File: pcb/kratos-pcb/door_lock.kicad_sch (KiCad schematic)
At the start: 8 parts, among them IC1 SN74HC595N, Q2 2N2222A, Q3 2N2222A, U2 74HC595

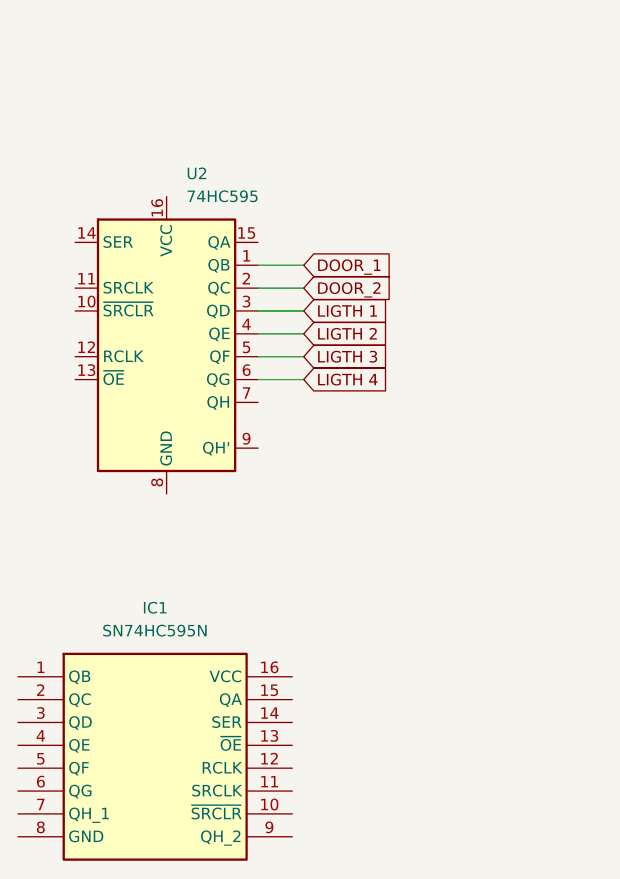
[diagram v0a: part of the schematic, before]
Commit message: ### added
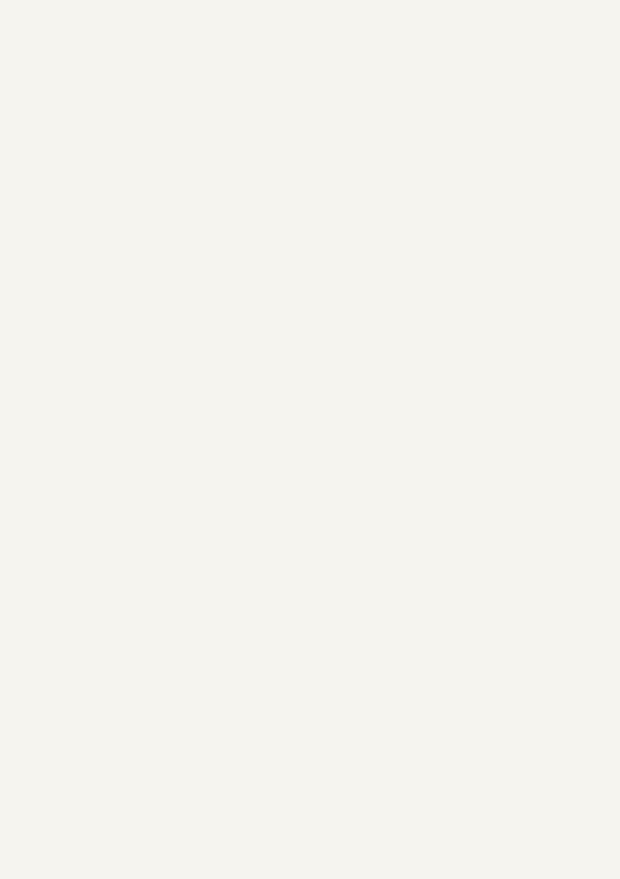
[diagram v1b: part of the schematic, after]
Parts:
- removed IC1: SN74HC595N, DIP794W53P254L1930H508Q16N, symbol SN74HC595N:SN74HC595N
- removed U2: 74HC595, symbol 74xx:74HC595

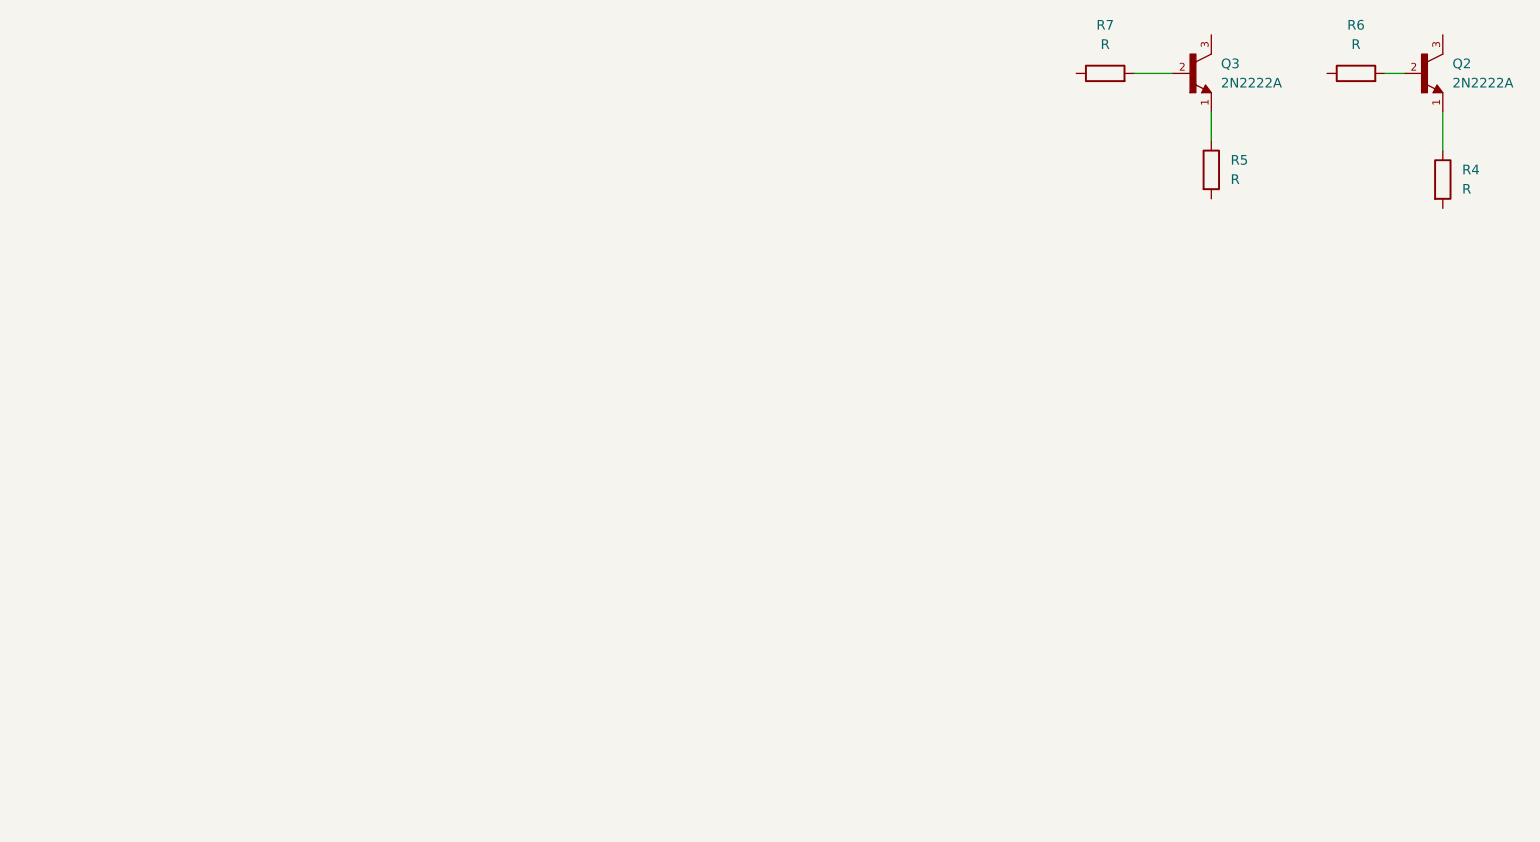
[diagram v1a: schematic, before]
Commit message: ### added
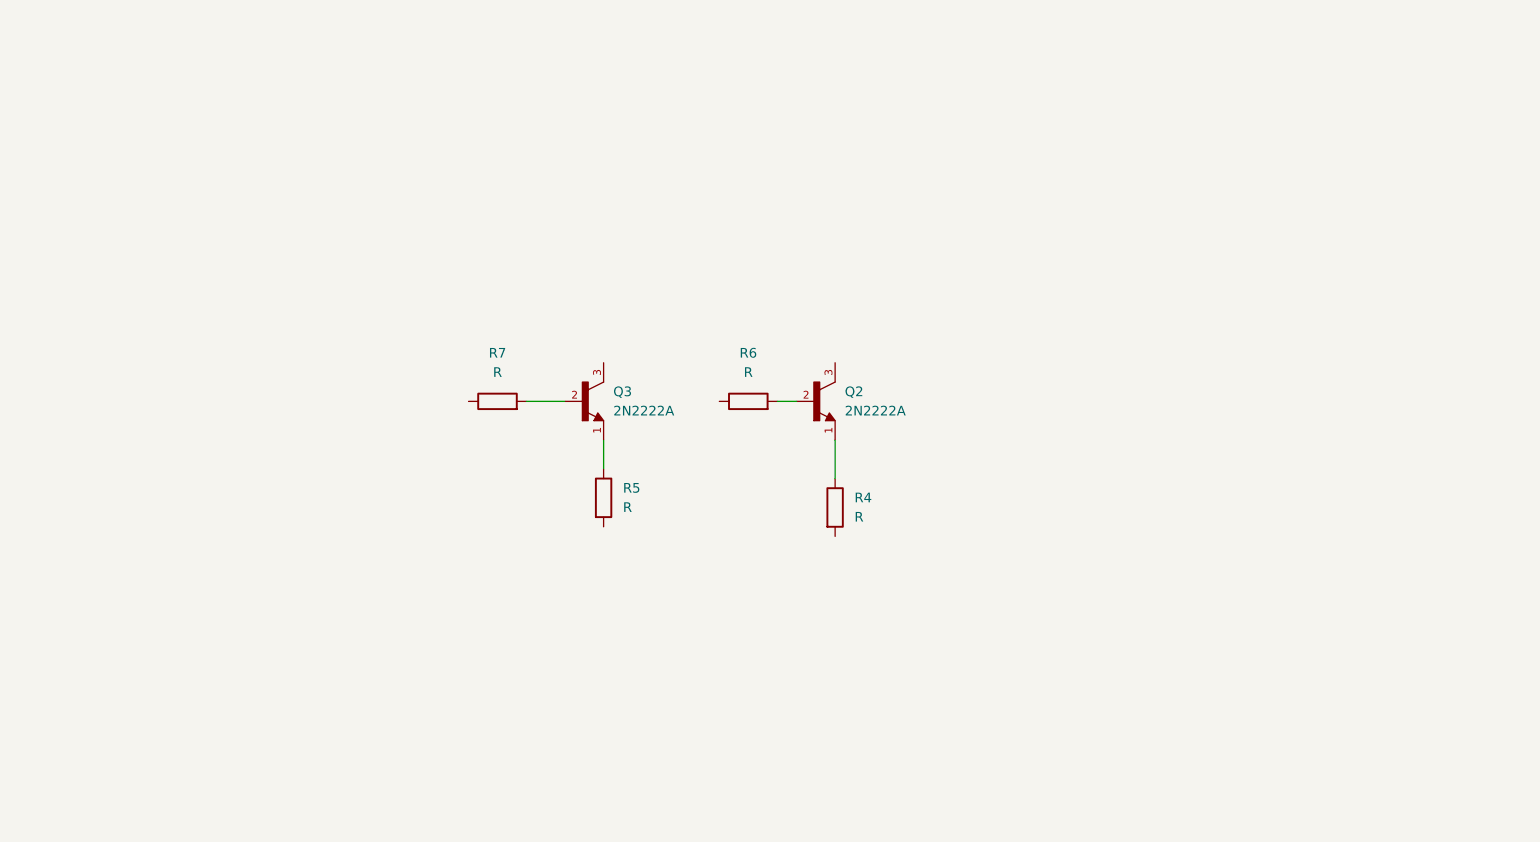
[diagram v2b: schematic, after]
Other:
- moved on the sheet: Q2, Q3, R4, R5, R6, R7

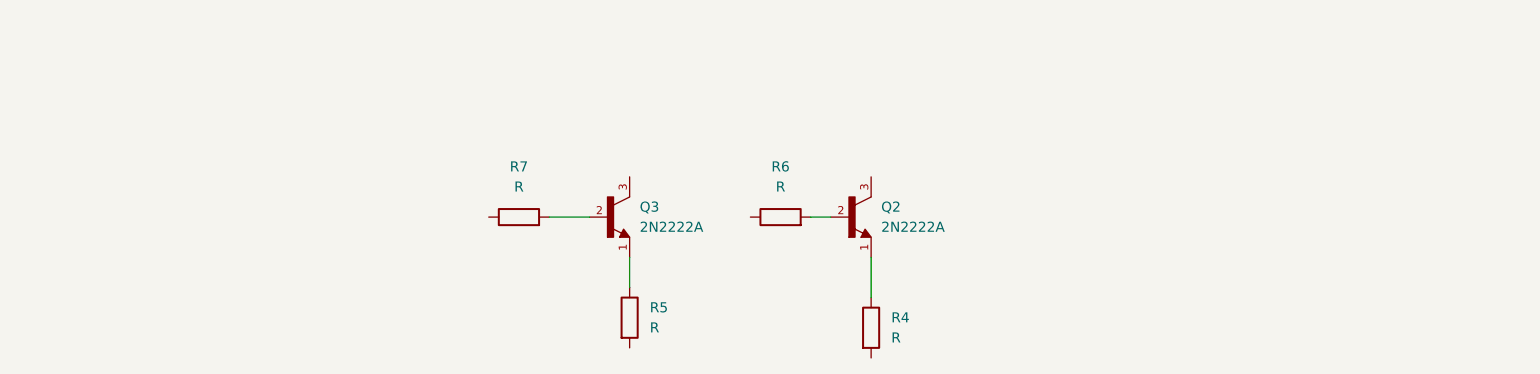
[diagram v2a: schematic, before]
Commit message: ### update     - kicad schematic
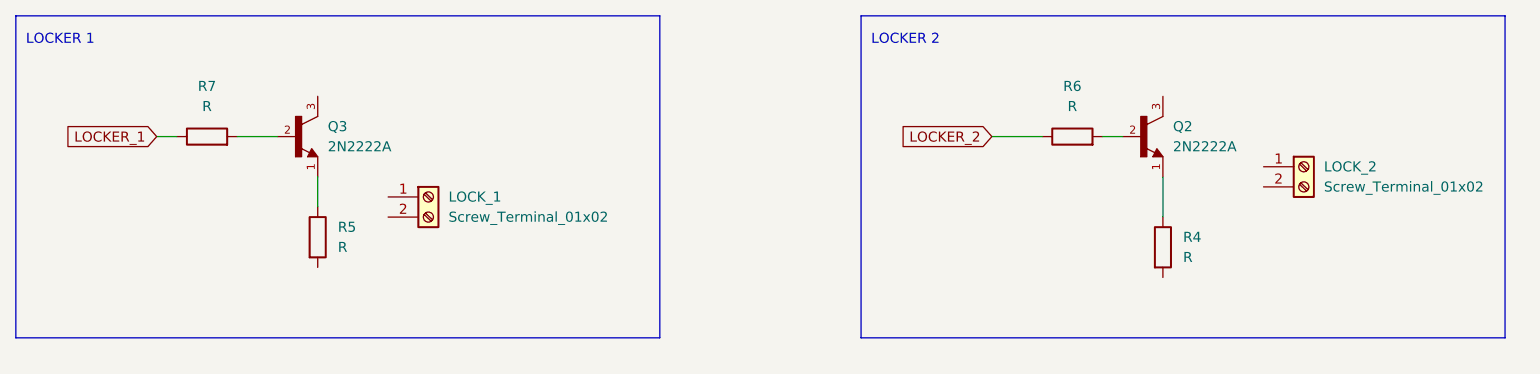
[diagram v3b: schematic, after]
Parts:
- added LOCK_1, LOCK_2: Screw_Terminal_01x02, TerminalBlock:TerminalBlock_bornier-2_P5.08mm, symbol Connector:Screw_Terminal_01x02
- R4, R5, R6, R7: footprint (none) -> Resistor_THT:R_Axial_DIN0204_L3.6mm_D1.6mm_P5.08mm_Horizontal
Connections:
- net LOCKER_2: now reaches R6.1
- net LOCKER_1: now reaches R7.1
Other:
- note added: "LOCKER 1"
- note added: "LOCKER 2"
- moved on the sheet: Q2, Q3, R4, R5, R6, R7

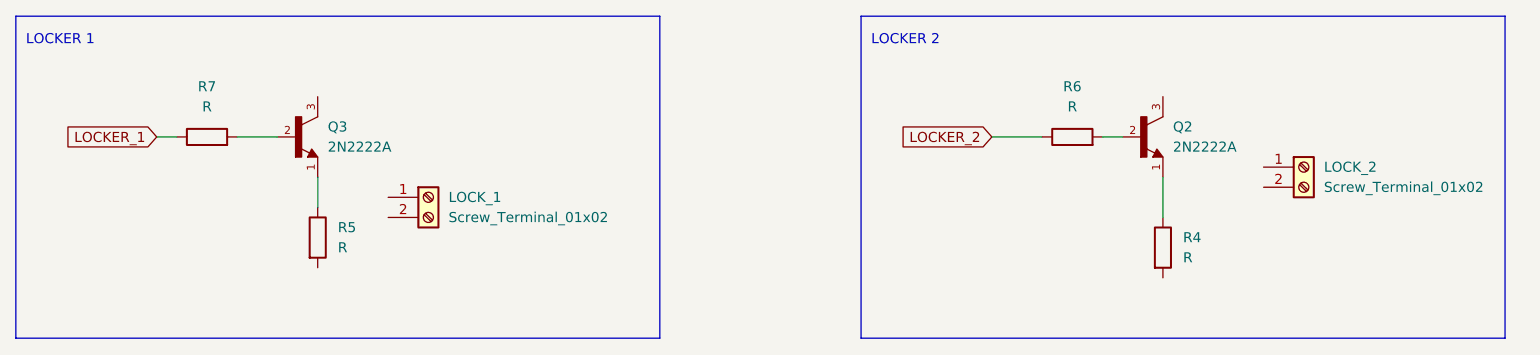
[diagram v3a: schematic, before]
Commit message: kicad
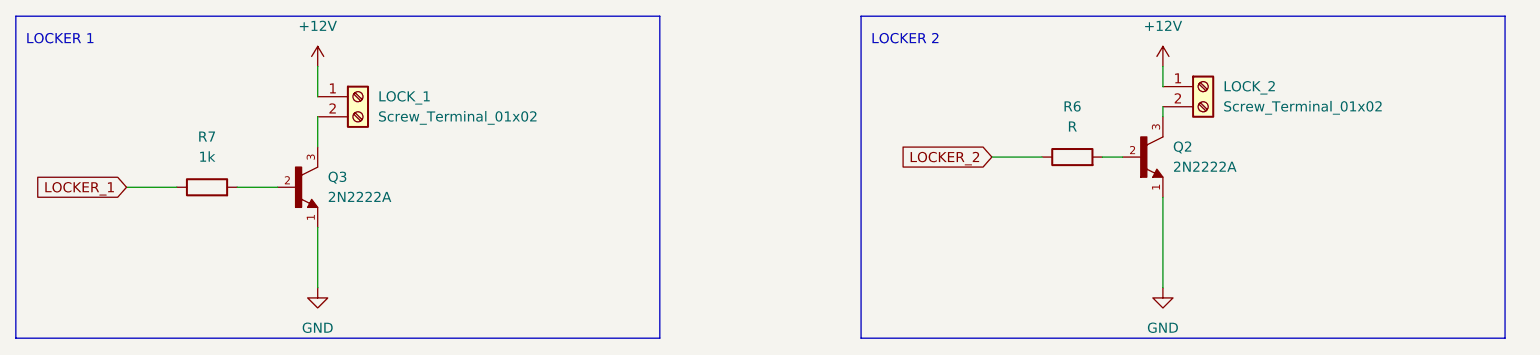
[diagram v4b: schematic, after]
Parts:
- removed R4, R5: R, Resistor_THT:R_Axial_DIN0204_L3.6mm_D1.6mm_P5.08mm_Horizontal, symbol Device:R
- R7: value R -> 1k
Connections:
- net GND: now reaches Q3.1
- net GND: now also Q2.1
- net at Q3.3: now also LOCK_1.2 (Pin_2)
- net at Q2.3: now also LOCK_2.2 (Pin_2)
- net +12V: now reaches LOCK_2.1 (Pin_1)
- net +12V: now also LOCK_1.1 (Pin_1)
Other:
- moved on the sheet: LOCK_1, LOCK_2, Q2, Q3, R6, R7

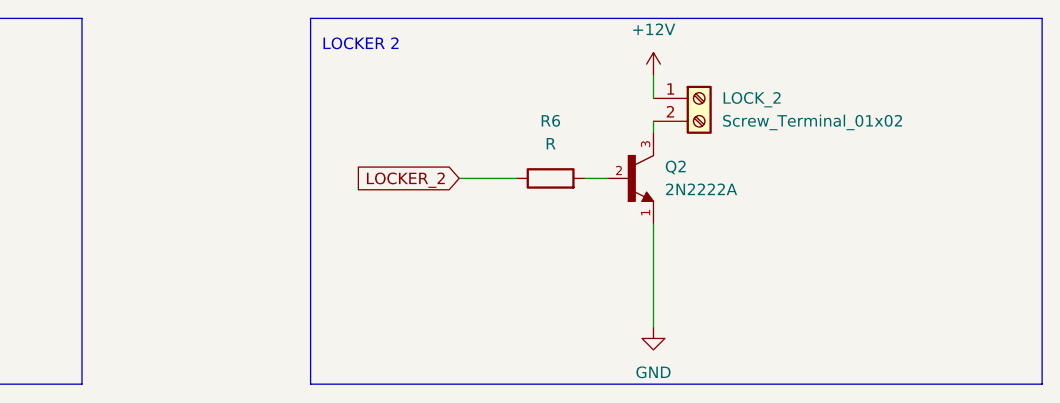
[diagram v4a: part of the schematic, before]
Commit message: ki
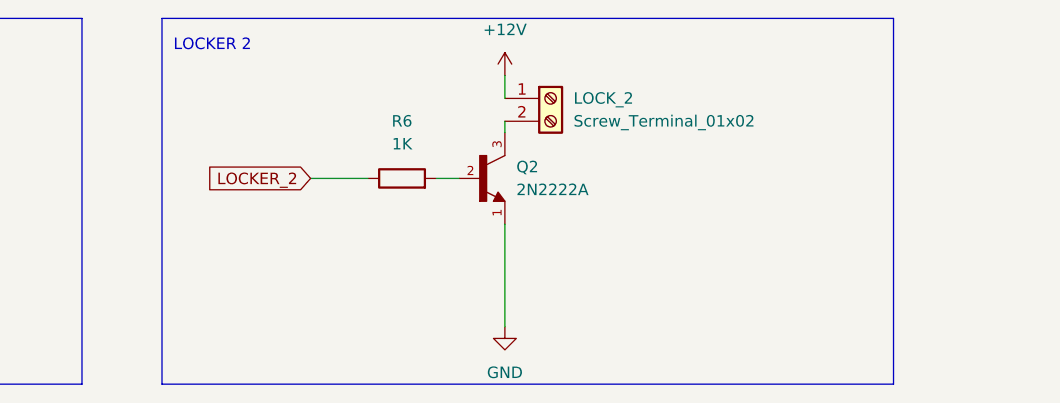
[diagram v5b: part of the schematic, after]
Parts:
- R6: value R -> 1K
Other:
- moved on the sheet: LOCK_2, Q2, R6
